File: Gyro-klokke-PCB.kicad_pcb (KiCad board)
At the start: 2 copper layers, 40.6 x 25.4 mm, 21 parts, among them J1 Conn_01x04_Male, J2 Conn_01x04_Male, J3 Conn_01x03_Male, J4 Conn_02x05_Odd_Even, SW1 SW_Push, SW2 SW_Push, U1 STM32F030F4Px, U2 LB1948MC, U3 LB1948MC, Y1 Crystal_Small

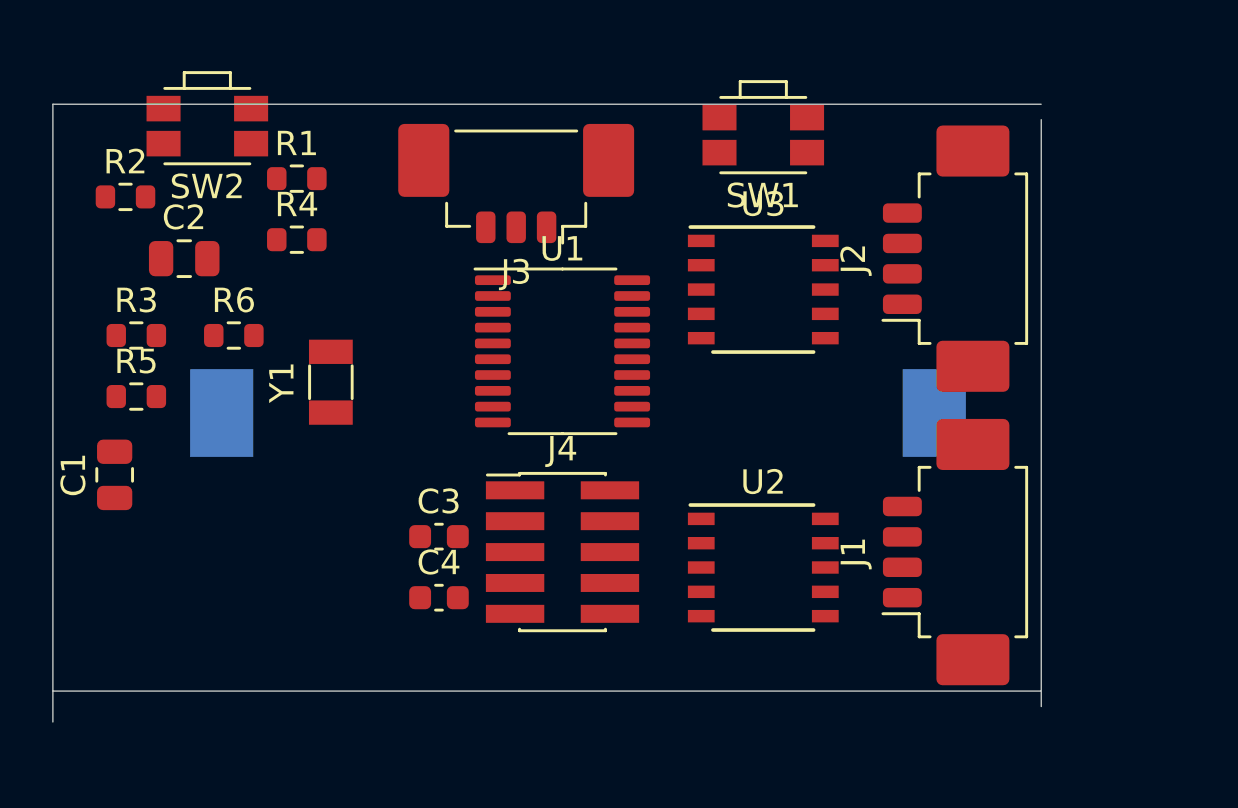
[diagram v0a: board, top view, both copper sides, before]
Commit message: Kretskort ferdig v1.0
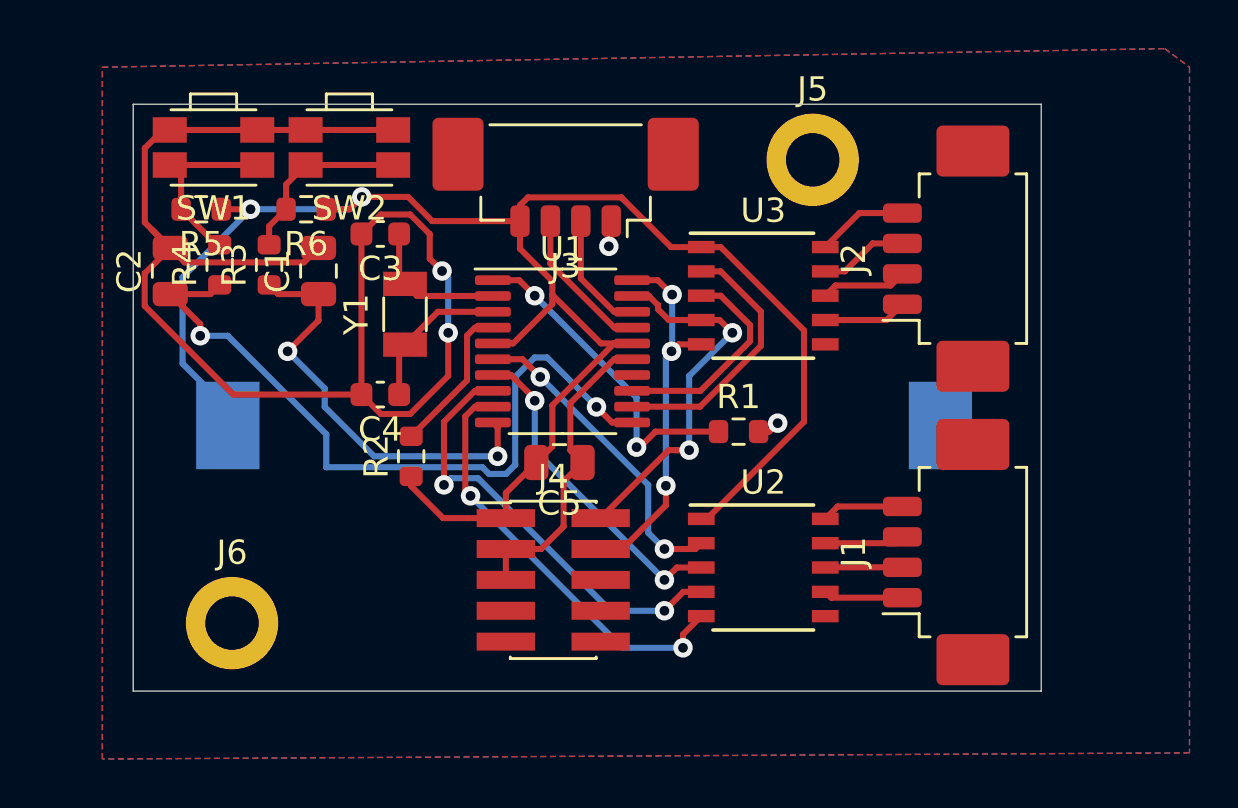
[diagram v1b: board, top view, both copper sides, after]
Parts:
- added C5: 100nF, Capacitor_SMD:C_0805_2012Metric, F.Cu at (174.5, 120.1)
- added J5: Conn_01x01_Female, MountingHole:MountingHole_2.2mm_M2_ISO14580_Pad, F.Cu at (184.9, 107.7)
- added J6: Conn_01x01_Female, MountingHole:MountingHole_2.2mm_M2_ISO14580_Pad, F.Cu at (161.0, 126.7)
- J3: footprint Connector_Molex:Molex_PicoBlade_53398-0371_1x03-1MP_P1.25mm_Vertical -> Connector_Molex:Molex_PicoBlade_53398-0471_1x04-1MP_P1.25mm_Vertical
- moved SW1 22.6 mm to (160.3, 107.2)
- moved R1 20.9 mm to (181.9, 118.9)
- moved R2 15.9 mm to (168.4, 119.9), turned to 90 degrees
- moved C3 12.7 mm to (167.1, 110.7), turned to 180 degrees
- moved C1 11.9 mm to (164.6, 112.3)
- moved C4 8.69 mm to (167.1, 117.3), turned to 180 degrees
- moved R5 8.15 mm to (159.8, 109.7), turned to 180 degrees
- moved R3 6.19 mm to (162.6, 112.0), turned to 90 degrees
- moved R6 5.98 mm to (164.1, 109.7), turned to 180 degrees
- moved SW2 5.91 mm to (165.9, 107.2)
- moved Y1 4.13 mm to (168.1, 114.0)
- moved R4 3.34 mm to (160.5, 112.0), turned to 90 degrees
- moved J3 2.05 mm to (174.8, 109.0)
- moved J4 1.20 mm to (174.2, 125.0)
- moved C2 0.77 mm to (158.5, 112.3), turned to 90 degrees
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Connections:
- J3 pad 2: uart-TX -> uart-RX
- J3 pad 3: +3V3 -> uart-TX
- SW1 pad 1: GNDREF -> Net-(R4-Pad2)
- SW1 pad 2: Net-(R4-Pad2) -> GNDREF
- U1 pad 18: (no net) -> uart-RX
- U2 pad 1: VCC -> +3V3
- U3 pad 1: VCC -> +3V3
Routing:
- net +3V3: track 0.00 -> 74.9 mm, vias 0 -> 2
- net GNDREF: track 0.00 -> 71.7 mm, vias 0 -> 4
- net Net-(C2-Pad1): track 0.00 -> 30.5 mm, vias 0 -> 2
- net mot1-B1: track 0.00 -> 18.4 mm, vias 0 -> 2
- net mot1-B2: track 0.00 -> 17.6 mm, vias 0 -> 2
- net Net-(C1-Pad1): track 0.00 -> 17.4 mm, vias 0 -> 2
- net SWD-SWIO: track 0.00 -> 15.8 mm, vias 0 -> 2
- net SWD-SWCLK: track 0.00 -> 15.4 mm, vias 0 -> 3
- net Net-(R1-Pad1): track 0.00 -> 13.6 mm, vias 0 -> 2
- net mot1-A2: track 0.00 -> 13.5 mm, vias 0 -> 2
- net mot1-A1: track 0.00 -> 13.1 mm, vias 0 -> 2
- net mot2-A1: track 0.00 -> 10.9 mm
- net mot2-A2: track 0.00 -> 8.86 mm
- net Net-(R4-Pad2): track 0.00 -> 7.81 mm
- net Net-(R3-Pad2): track 0.00 -> 7.50 mm
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- added copper zone on B.Cu, net GNDREF
- added copper zone on F.Cu, net GNDREF
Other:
- board size 40.6 x 25.4 mm -> 37.3 x 24.1 mm
